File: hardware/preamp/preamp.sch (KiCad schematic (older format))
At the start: 18 parts, among them J1 I/O, J4 Coil, U1 TLV170DBV

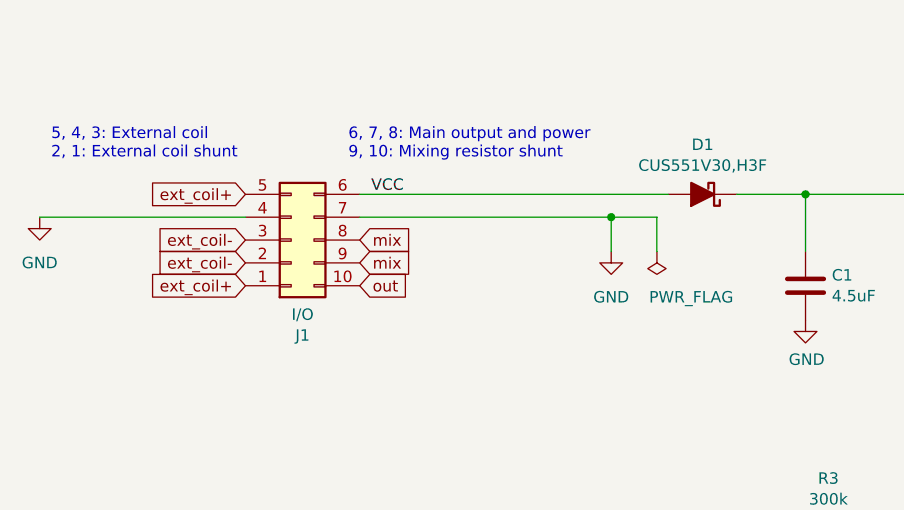
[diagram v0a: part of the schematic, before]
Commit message: preamp updates/minor tweaks
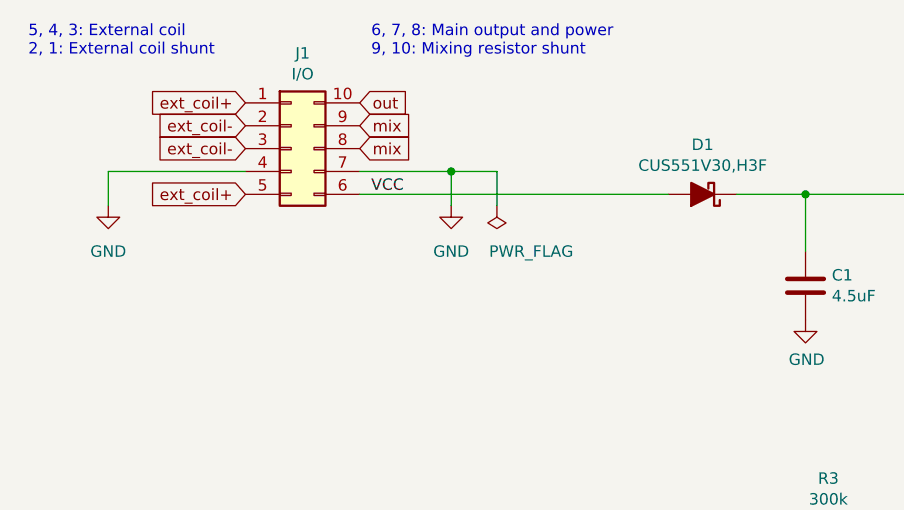
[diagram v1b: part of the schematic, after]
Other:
- moved on the sheet: J1
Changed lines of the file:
@@
 	1    0    0    -1
-$EndComp
-$Comp
-L Device:D_Schottky_ALT D1
-U 1 1 60CC8B99
-P 5350 2100
-F 0 "D1" H 5350 1883 50  0000 C CNN
-F 1 "CUS551V30,H3F" H 5350 1974 50  0000 C CNN
-F 2 "Diode_SMD:D_SOD-323" H 5350 2100 50  0001 C CNN
-F 3 "~" H 5350 2100 50  0001 C CNN
-	1    5350 2100
-	-1   0    0    1
 $EndComp
 Text GLabel 3350 4200 0    50   Input ~ 0
@@
 	1    0    0    -1
 $EndComp
-$Comp
-L power:GND #PWR0106
-U 1 1 60CDB5FB
-P 4950 2350
-F 0 "#PWR0106" H 4950 2100 50  0001 C CNN
-F 1 "GND" H 4950 2150 50  0000 C CNN
-F 2 "" H 4950 2350 50  0001 C CNN
-F 3 "" H 4950 2350 50  0001 C CNN
-	1    4950 2350
-	1    0    0    -1
-$EndComp
-Wire Wire Line
-	4950 2200 4950 2350
-$Comp
-L power:PWR_FLAG #FLG02
-U 1 1 60D52BC1
-P 5150 2350
-F 0 "#FLG02" H 5150 2425 50  0001 C CNN
-F 1 "PWR_FLAG" H 5000 2550 50  0000 C CNN
-F 2 "" H 5150 2350 50  0001 C CNN
-F 3 "~" H 5150 2350 50  0001 C CNN
-	1    5150 2350
-	-1   0    0    1
-$EndComp
-Wire Wire Line
-	5150 2350 5150 2200
-Wire Wire Line
-	5150 2200 4950 2200
-Text Notes 3800 1950 0    50   ~ 0
+Text Notes 3900 1500 0    50   ~ 0
 6, 7, 8: Main output and power\n9, 10: Mixing resistor shunt
-Text Notes 2500 1950 0    50   ~ 0
+Text Notes 2400 1500 0    50   ~ 0
 5, 4, 3: External coil\n2, 1: External coil shunt
-$Comp
-L Connector_Generic:Conn_02x05_Counter_Clockwise J1
-U 1 1 60CB8C21
-P 3550 2300
-F 0 "J1" H 3600 2717 50  0000 C CNN
-F 1 "I/O" H 3600 2626 50  0000 C CNN
-F 2 "cycfi_library:pin_header_2x5p_2.54mm_smd_horizontal" H 3550 2300 50  0001 C CNN
-F 3 "~" H 3550 2300 50  0001 C CNN
-	1    3550 2300
-	1    0    0    1
-$EndComp
 $Comp
 L power:GND #PWR0107
 U 1 1 60CC841D
-P 2450 2200
-F 0 "#PWR0107" H 2450 1950 50  0001 C CNN
-F 1 "GND" H 2450 2000 50  0000 C CNN
-F 2 "" H 2450 2200 50  0001 C CNN
-F 3 "" H 2450 2200 50  0001 C CNN
-	1    2450 2200
+P 2750 2150
+F 0 "#PWR0107" H 2750 1900 50  0001 C CNN
+F 1 "GND" H 2750 1950 50  0000 C CNN
+F 2 "" H 2750 2150 50  0001 C CNN
+F 3 "" H 2750 2150 50  0001 C CNN
+	1    2750 2150
 	1    0    0    -1
 $EndComp
-Text GLabel 3850 2500 2    50   Input ~ 0
+Text GLabel 3850 1700 2    50   Input ~ 0
 out
-Text GLabel 3850 2400 2    50   Input ~ 0
+Text GLabel 3850 1800 2    50   Input ~ 0
 mix
-Text GLabel 3850 2300 2    50   Input ~ 0
+Text GLabel 3850 1900 2    50   Input ~ 0
 mix
 Text GLabel 3350 2100 0    50   Input ~ 0
 ext_coil+
-Text GLabel 3350 2300 0    50   Input ~ 0
+Text GLabel 3350 1900 0    50   Input ~ 0
 ext_coil-
-Text GLabel 3350 2400 0    50   Input ~ 0
+Text GLabel 3350 1800 0    50   Input ~ 0
 ext_coil-
-Text GLabel 3350 2500 0    50   Input ~ 0
+Text GLabel 3350 1700 0    50   Input ~ 0
 ext_coil+
 $Comp
@@
 Wire Wire Line
 	5200 2100 3850 2100
-Wire Wire Line
-	3850 2200 4950 2200
-Connection ~ 4950 2200
-Wire Wire Line
-	3350 2200 2450 2200
 Text Label 3900 2100 0    50   ~ 0
 VCC
@@
 Wire Wire Line
 	8750 4550 8950 4550
+$Comp
+L Connector_Generic:Conn_02x05_Counter_Clockwise J1
+U 1 1 60CB8C21
+P 3550 1900
+F 0 "J1" H 3600 2317 50  0000 C CNN
+F 1 "I/O" H 3600 2226 50  0000 C CNN
+F 2 "cycfi_library:pin_header_2x5p_2.54mm_smd_horizontal" H 3550 1900 50  0001 C CNN
+F 3 "~" H 3550 1900 50  0001 C CNN
+	1    3550 1900
+	1    0    0    -1
+$EndComp
+$Comp
+L power:PWR_FLAG #FLG02
+U 1 1 60D52BC1
+P 4450 2150
+F 0 "#FLG02" H 4450 2225 50  0001 C CNN
+F 1 "PWR_FLAG" H 4300 2350 50  0000 C CNN
+F 2 "" H 4450 2150 50  0001 C CNN
+F 3 "~" H 4450 2150 50  0001 C CNN
+	1    4450 2150
+	-1   0    0    1
+$EndComp
+$Comp
+L power:GND #PWR0106
+U 1 1 60CDB5FB
+P 4250 2150
+F 0 "#PWR0106" H 4250 1900 50  0001 C CNN
+F 1 "GND" H 4250 1950 50  0000 C CNN
+F 2 "" H 4250 2150 50  0001 C CNN
+F 3 "" H 4250 2150 50  0001 C CNN
+	1    4250 2150
+	1    0    0    -1
+$EndComp
+$Comp
+L Device:D_Schottky_ALT D1
+U 1 1 60CC8B99
+P 5350 2100
+F 0 "D1" H 5350 1883 50  0000 C CNN
+F 1 "CUS551V30,H3F" H 5350 1974 50  0000 C CNN
+F 2 "Diode_SMD:D_SOD-323" H 5350 2100 50  0001 C CNN
+F 3 "~" H 5350 2100 50  0001 C CNN
+	1    5350 2100
+	-1   0    0    1
+$EndComp
+Wire Wire Line
+	4250 2000 3850 2000
+Wire Wire Line
+	4450 2150 4450 2000
+Wire Wire Line
+	4450 2000 4250 2000
+Connection ~ 4250 2000
+Wire Wire Line
+	4250 2150 4250 2000
+Wire Wire Line
+	2750 2000 2750 2150
+Wire Wire Line
+	3350 2000 2750 2000
 $EndSCHEMATC

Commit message: Preamp updates
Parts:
- H1, H2, H3, H4: footprint cycfi_library:mounting_hole_2.1mm -> cycfi_library:mounting_hole_st1.9
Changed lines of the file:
@@
 Wire Wire Line
 	8200 3950 8500 3950
-$Comp
-L Mechanical:MountingHole H1
-U 1 1 60CC8E41
-P 8300 2100
-F 0 "H1" H 8400 2146 50  0000 L CNN
-F 1 "MountingHole" H 8400 2055 50  0000 L CNN
-F 2 "cycfi_library:mounting_hole_2.1mm" H 8300 2100 50  0001 C CNN
-F 3 "~" H 8300 2100 50  0001 C CNN
-	1    8300 2100
-	1    0    0    -1
-$EndComp
-$Comp
-L Mechanical:MountingHole H2
-U 1 1 60CC94F0
-P 8300 2300
-F 0 "H2" H 8400 2346 50  0000 L CNN
-F 1 "MountingHole" H 8400 2255 50  0000 L CNN
-F 2 "cycfi_library:mounting_hole_2.1mm" H 8300 2300 50  0001 C CNN
-F 3 "~" H 8300 2300 50  0001 C CNN
-	1    8300 2300
-	1    0    0    -1
-$EndComp
-$Comp
-L Mechanical:MountingHole H3
-U 1 1 60CCA720
-P 8300 2500
-F 0 "H3" H 8400 2546 50  0000 L CNN
-F 1 "MountingHole" H 8400 2455 50  0000 L CNN
-F 2 "cycfi_library:mounting_hole_2.1mm" H 8300 2500 50  0001 C CNN
-F 3 "~" H 8300 2500 50  0001 C CNN
-	1    8300 2500
-	1    0    0    -1
-$EndComp
-$Comp
-L Mechanical:MountingHole H4
-U 1 1 60CCABB9
-P 8300 2700
-F 0 "H4" H 8400 2746 50  0000 L CNN
-F 1 "MountingHole" H 8400 2655 50  0000 L CNN
-F 2 "cycfi_library:mounting_hole_2.1mm" H 8300 2700 50  0001 C CNN
-F 3 "~" H 8300 2700 50  0001 C CNN
-	1    8300 2700
-	1    0    0    -1
-$EndComp
 Text Notes 3900 1500 0    50   ~ 0
 6, 7, 8: Main output and power\n9, 10: Mixing resistor shunt
@@
 Wire Wire Line
 	3350 2000 2750 2000
+$Comp
+L Mechanical:MountingHole H4
+U 1 1 60CCABB9
+P 8300 2700
+F 0 "H4" H 8400 2746 50  0000 L CNN
+F 1 "MountingHole" H 8400 2655 50  0000 L CNN
+F 2 "cycfi_library:mounting_hole_st1.9" H 8300 2700 50  0001 C CNN
+F 3 "~" H 8300 2700 50  0001 C CNN
+	1    8300 2700
+	1    0    0    -1
+$EndComp
+$Comp
+L Mechanical:MountingHole H3
+U 1 1 60CCA720
+P 8300 2500
+F 0 "H3" H 8400 2546 50  0000 L CNN
+F 1 "MountingHole" H 8400 2455 50  0000 L CNN
+F 2 "cycfi_library:mounting_hole_st1.9" H 8300 2500 50  0001 C CNN
+F 3 "~" H 8300 2500 50  0001 C CNN
+	1    8300 2500
+	1    0    0    -1
+$EndComp
+$Comp
+L Mechanical:MountingHole H2
+U 1 1 60CC94F0
+P 8300 2300
+F 0 "H2" H 8400 2346 50  0000 L CNN
+F 1 "MountingHole" H 8400 2255 50  0000 L CNN
+F 2 "cycfi_library:mounting_hole_st1.9" H 8300 2300 50  0001 C CNN
+F 3 "~" H 8300 2300 50  0001 C CNN
+	1    8300 2300
+	1    0    0    -1
+$EndComp
+$Comp
+L Mechanical:MountingHole H1
+U 1 1 60CC8E41
+P 8300 2100
+F 0 "H1" H 8400 2146 50  0000 L CNN
+F 1 "MountingHole" H 8400 2055 50  0000 L CNN
+F 2 "cycfi_library:mounting_hole_st1.9" H 8300 2100 50  0001 C CNN
+F 3 "~" H 8300 2100 50  0001 C CNN
+	1    8300 2100
+	1    0    0    -1
+$EndComp
 $EndSCHEMATC
